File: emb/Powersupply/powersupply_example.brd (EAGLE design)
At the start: 101.3 x 76.2 mm, 15 parts, among them IC1 7805TV, IC2 7812TV, IC3 LM2574N-5.0

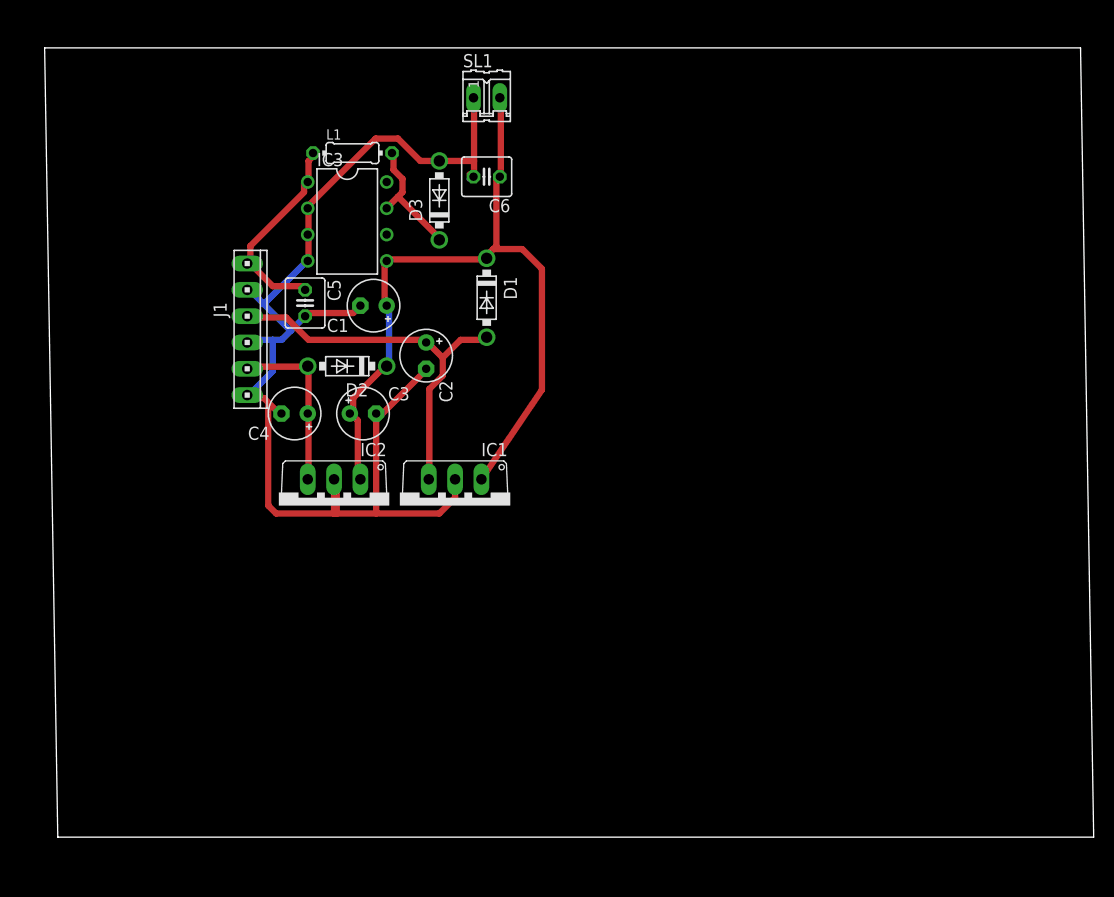
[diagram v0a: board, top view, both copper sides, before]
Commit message: Updated PCB board
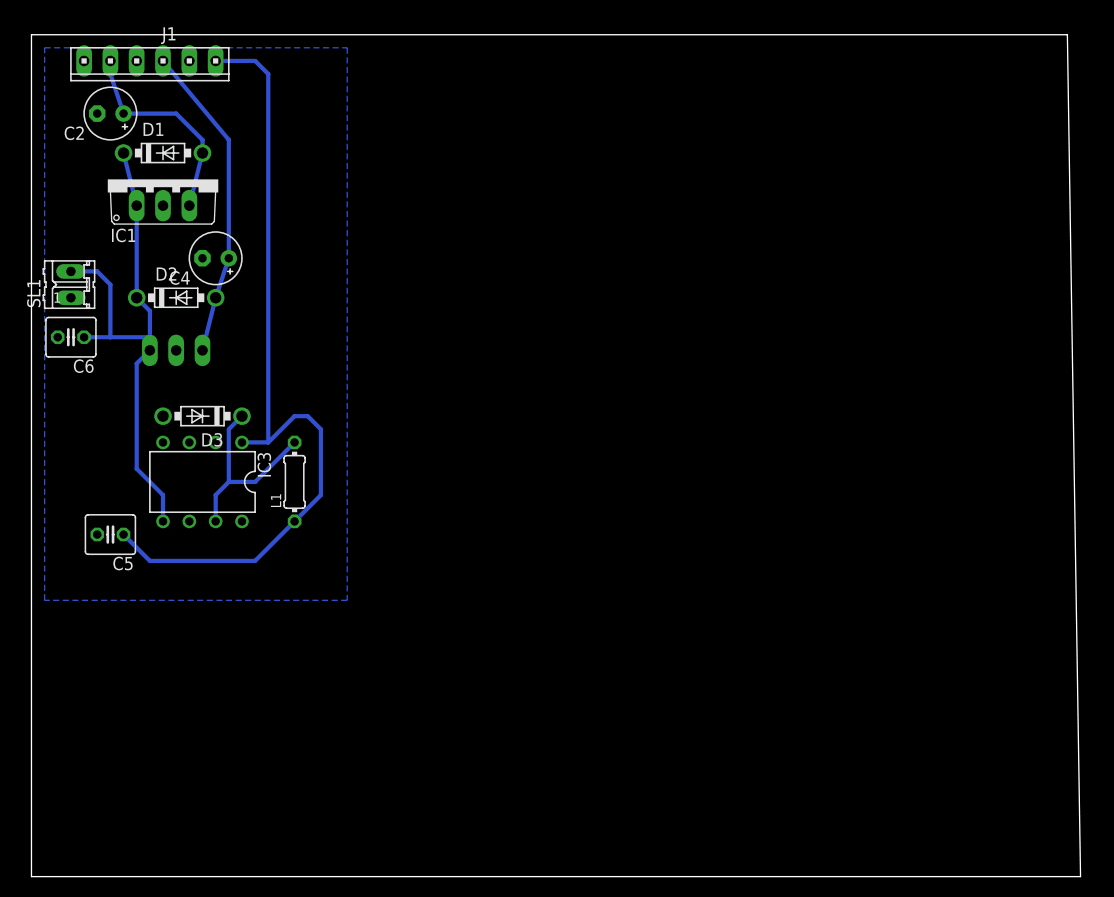
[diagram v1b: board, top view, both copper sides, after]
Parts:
- removed C1, C3: 22µF, rcl:E2,5-5
- moved SL1 44.0 mm to (2.54, 57.1), turned to 90 degrees
- moved C6 43.0 mm to (2.54, 52.1)
- moved IC1 42.3 mm to (11.4, 67.3), turned to 0 degrees
- moved C2 38.4 mm to (6.35, 73.7), turned to 180 degrees
- moved D1 34.2 mm to (11.4, 69.8), turned to 0 degrees
- moved L1 32.2 mm to (24.1, 38.1), turned to 90 degrees
- moved D3 30.9 mm to (15.2, 44.5), turned to 180 degrees
- moved C5 29.2 mm to (6.35, 33.0), turned to 180 degrees
- moved IC3 28.8 mm to (15.2, 38.1), turned to 180 degrees
- moved J1 27.6 mm to (10.2, 78.7), turned to 180 degrees
- moved IC2 19.7 mm to (12.7, 48.3), flipped to the bottom
- moved D2 17.8 mm to (12.7, 55.9), turned to 0 degrees
- moved C4 16.8 mm to (16.5, 59.7)
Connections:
- net 12V: now also J1.4; no longer J1.2
- net 15V: no longer C1.+, C3.+
- net 6V: now also J1.2; no longer J1.4
- net GND: no longer C1.-, C3.-
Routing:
- net GND: track 75.5 -> 0.00 mm
- net 5V: track 20.1 -> 79.4 mm
- net N$1: track 38.4 -> 0.00 mm
- net 15V: track 77.0 -> 53.6 mm
- net 6V: track 37.9 -> 20.5 mm
- net 12V: track 16.9 -> 30.6 mm
- net N$2: track 10.3 -> 0.00 mm
- net N$4: track 12.4 -> 19.1 mm
- added copper zone on layer 16, net GND
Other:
- board size 101.3 x 76.2 mm -> 101.3 x 81.3 mm
